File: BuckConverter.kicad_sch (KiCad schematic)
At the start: 10 parts, among them U1 TPS56339DDC

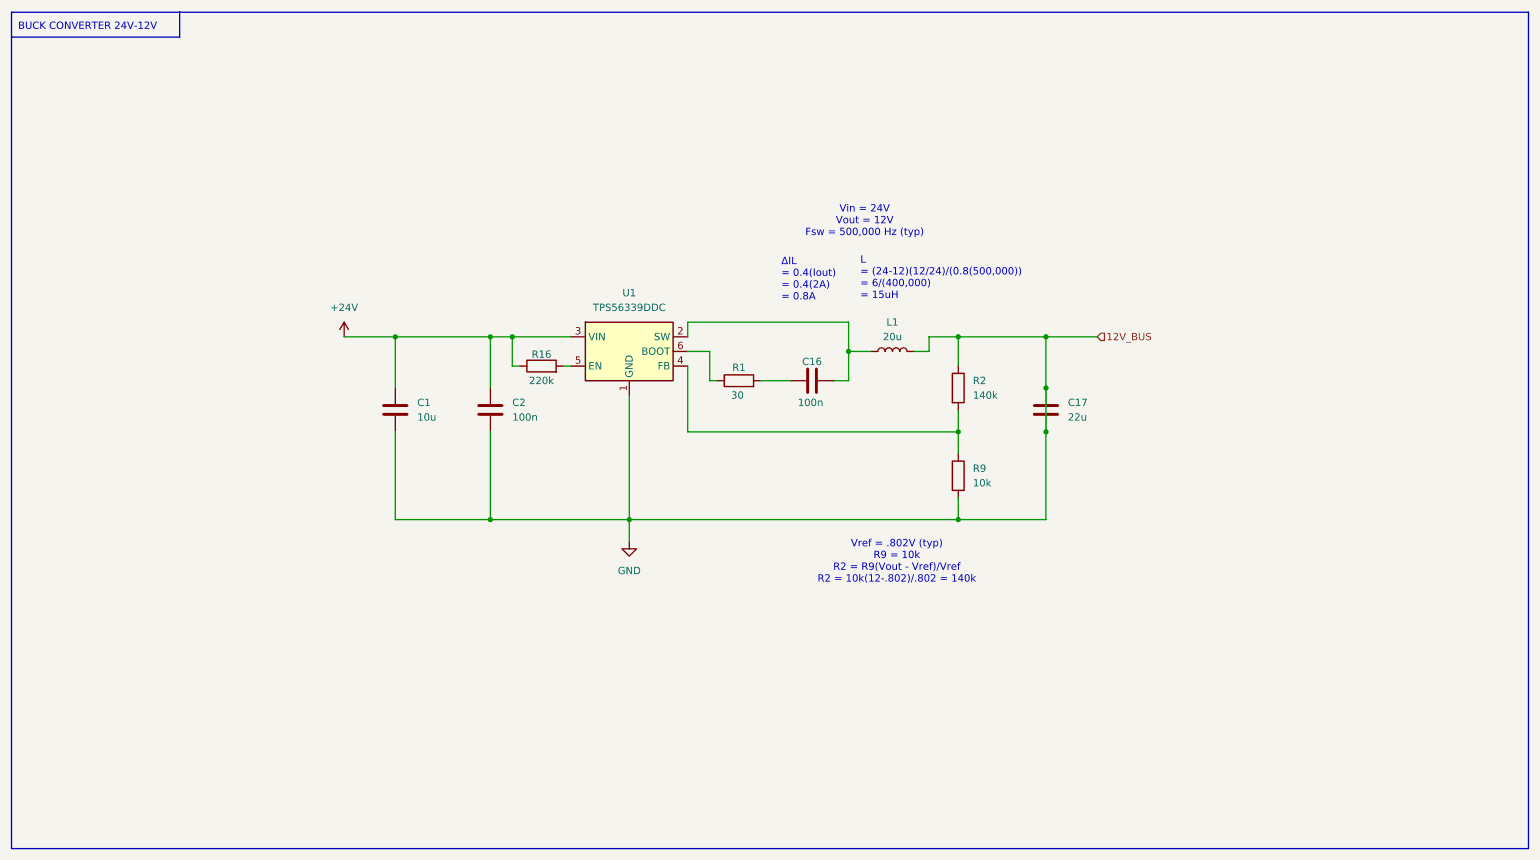
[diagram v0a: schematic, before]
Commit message: changes + ioc
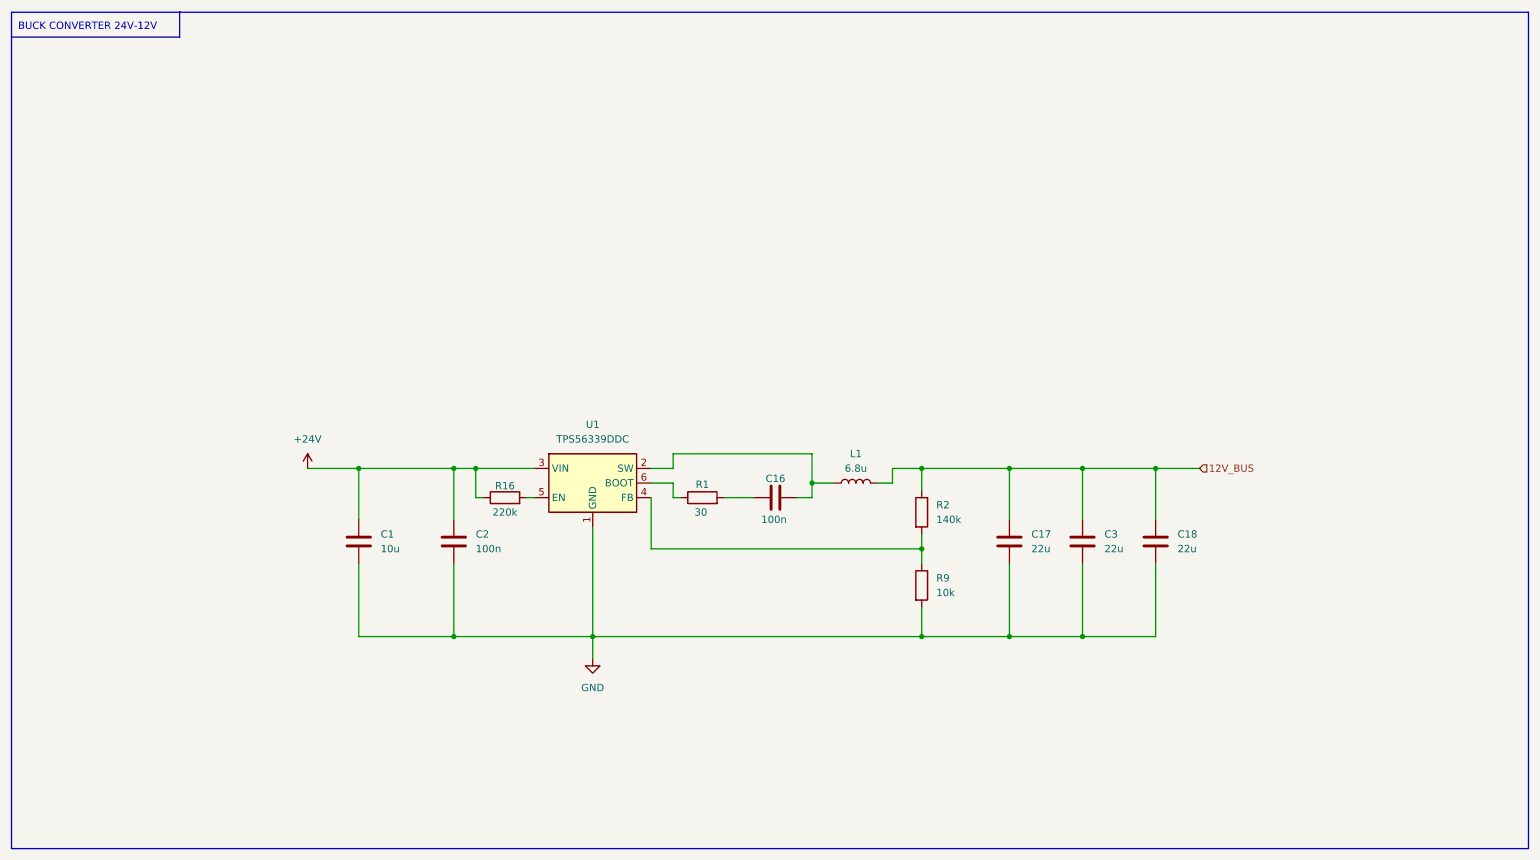
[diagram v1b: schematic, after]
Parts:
- added C18, C3: 22u, symbol Device:C
- L1: value 20u -> 6.8u
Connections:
- net GND: now also C18.2, C3.2; no longer C17.1, L1.2, R2.1
- new net 12V_BUS: C17.1, C18.1, C3.1, L1.2, R2.1
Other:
- note removed: "L = (24-12)(12/24)/(0.8(500,000)) = 6/(400,000) = 15uH"
- note removed: "Vin = 24V Vout = 12V Fsw = 500,000 Hz (typ)"
- note removed: "Vref = .802V (typ) R9 = 10k R2 = R9(Vout - Vref)/Vref R2 = 10k(12-.802)/.802 = 140k"
- note removed: "ΔIL = 0.4(Iout) = 0.4(2A) = 0.8A"
- moved on the sheet: C1, C16, C17, C2, L1, R1, R16, R2, R9, U1
